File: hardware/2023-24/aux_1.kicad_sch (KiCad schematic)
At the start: 25 parts, among them J3 Screw_Terminal_01x04, Q5 BC817, U4 LM5066

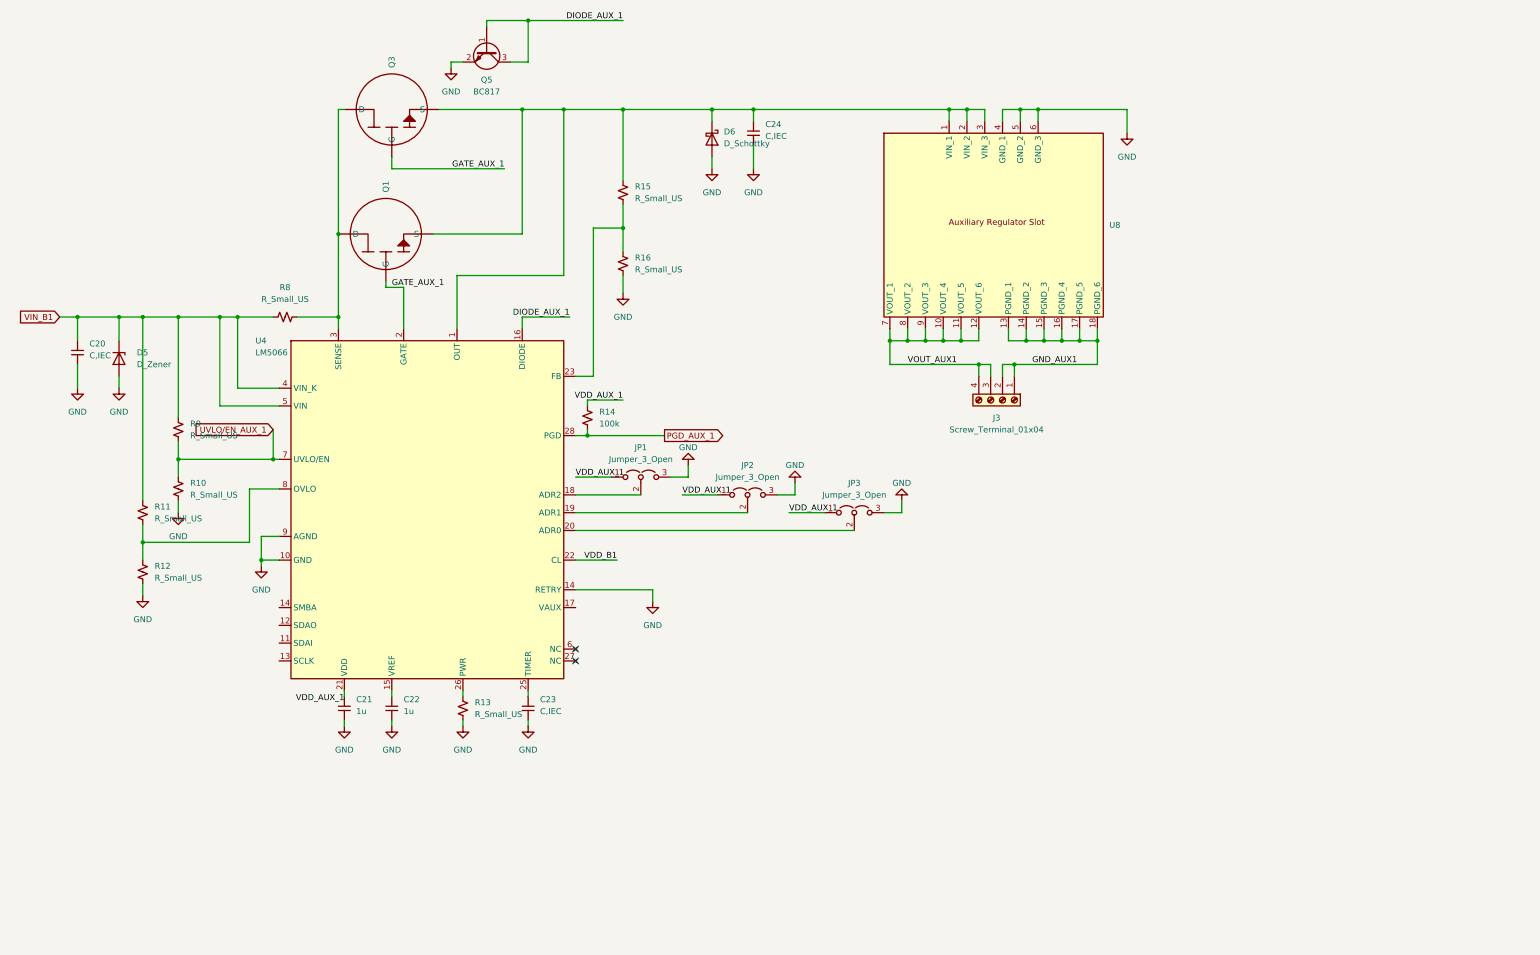
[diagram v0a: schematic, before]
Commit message: Pushing for design review
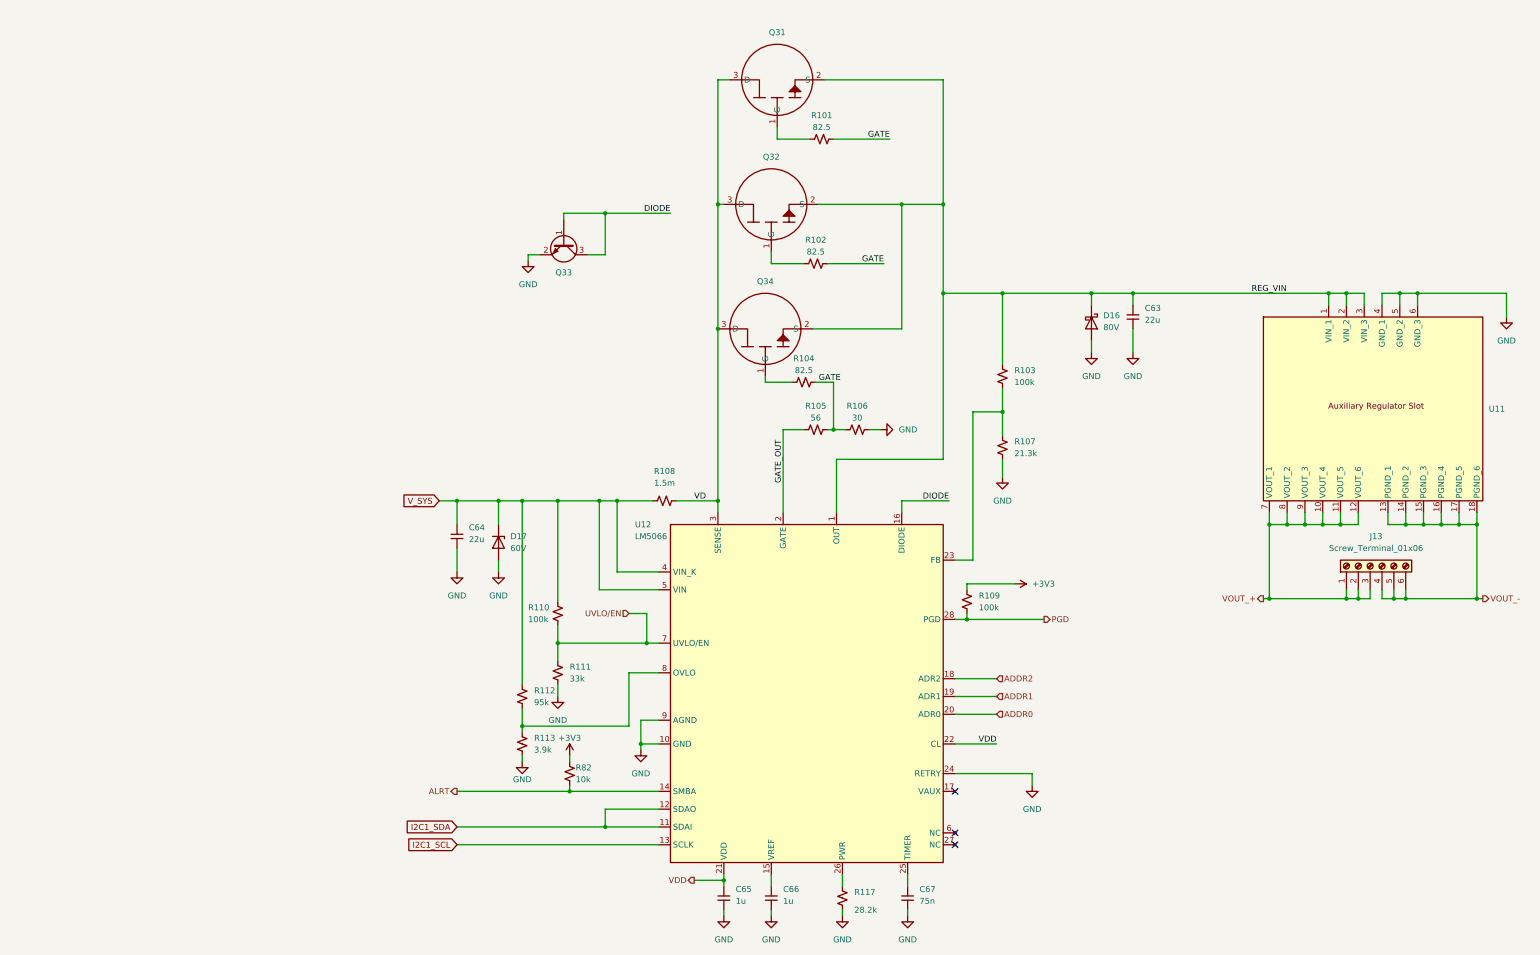
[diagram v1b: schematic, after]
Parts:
- removed C24: C,IEC, symbol PCM_Generic-50:C,IEC
- removed D5: D_Zener, symbol Device:D_Zener
- removed D6: D_Schottky, symbol Device:D_Schottky
- removed J3: Screw_Terminal_01x04, TerminalBlock:TerminalBlock_bornier-4_P5.08mm, symbol Connector:Screw_Terminal_01x04
- removed JP1, JP2, JP3: Jumper_3_Open, symbol Jumper:Jumper_3_Open
- removed Q5: BC817, Package_TO_SOT_SMD:SOT-23, symbol Transistor_BJT:BC817
- removed R10, R11, R12, R15, R16, R9: R_Small_US, symbol Device:R_Small_US
- added C63: 22u, Capacitor_SMD:CP_Elec_8x10, symbol PCM_Generic-50:C,IEC
- added D16: 80V, Diode_SMD:D_SMC, symbol Device:D_Schottky
- added D17: 60V, Diode_SMD:D_SMC, symbol Device:D_Zener
- added J13: Screw_Terminal_01x06, TerminalBlock_Phoenix:TerminalBlock_Phoenix_MKDS-1,5-6-5.08_1x06_P5.08mm_Horizontal, symbol Connector:Screw_Terminal_01x06
- added Q31: ~, Nexperia:WLCSP-8, symbol Nexperia:GAN3R2-100CBE
- added Q33: ~, Package_TO_SOT_SMD:SOT-23, symbol Transistor_BJT:BC817
- added R101, R102, R104: 82.5, Resistor_SMD:R_0603_1608Metric, symbol Device:R_Small_US
- added R103, R110: 100k, Resistor_SMD:R_0603_1608Metric, symbol Device:R_Small_US
- added R105: 56, Resistor_SMD:R_2512_6332Metric, symbol Device:R_Small_US
- added R106: 30, Resistor_SMD:R_2512_6332Metric, symbol Device:R_Small_US
- added R107: 21.3k, Resistor_SMD:R_0603_1608Metric, symbol Device:R_Small_US
- added R111: 33k, Resistor_SMD:R_0603_1608Metric, symbol Device:R_Small_US
- added R112: 95k, Resistor_SMD:R_0603_1608Metric, symbol Device:R_Small_US
- added R113: 3.9k, Resistor_SMD:R_0603_1608Metric, symbol Device:R_Small_US
- added R82: 10k, Resistor_SMD:R_0603_1608Metric, symbol Device:R_Small_US
- C64: renamed from C20; value C,IEC -> 22u; footprint (none) -> Capacitor_SMD:CP_Elec_8x10; MPN (none) -> EEE-FK2A220V
- C65: renamed from C21; footprint (none) -> Capacitor_SMD:C_0603_1608Metric
- C66: renamed from C22; footprint (none) -> Capacitor_SMD:C_0603_1608Metric
- C67: renamed from C23; value C,IEC -> 75n; footprint (none) -> Capacitor_SMD:C_0402_1005Metric; MPN (none) -> GRM31C5C1H753JA01L
- Q32: renamed from Q3; symbol Nexperia:GAN3R2-100CBEAZ -> Nexperia:GAN3R2-100CBE
- Q34: renamed from Q1; symbol Nexperia:GAN3R2-100CBEAZ -> Nexperia:GAN3R2-100CBE
- R108: renamed from R8; value R_Small_US -> 1.5m; footprint (none) -> Resistor_SMD:R_2512_6332Metric; MPN (none) -> WSL25121L500FEA; Manufacturer (none) -> Vishay
- R109: renamed from R14; footprint (none) -> Resistor_SMD:R_0603_1608Metric
- R117: renamed from R13; value R_Small_US -> 28.2k; footprint (none) -> Resistor_SMD:R_0603_1608Metric
- renumbered U8 to U11, U4 to U12
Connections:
- net VDD_B1 is gone; now on net VDD: U12.22 (CL)
- net GND: now also U12.24 (RETRY), C63.2 (-), D16.2 (A), D17.2 (A), Q33.2 (E), R106.2, R107.2, R111.1, R113.1; no longer U12.14 (SMBA)
- net VDD: now reaches C65.1 (+), U12.21 (VDD)
- net at U12.8 (OVLO): now also R112.1, R113.2
- net REG_VIN: now reaches U11.1 (VIN_1), U11.2 (VIN_2), U11.3 (VIN_3), U12.1 (OUT)
- net REG_VIN: now also Q32.2 (S), Q34.2 (S), C63.1 (+), D16.1 (K), Q31.2 (S), R103.1; no longer Q32. (S), Q34. (S)
- net I2C1_SDA: now reaches U12.11 (SDAI)
- net I2C1_SDA: now also U12.12 (SDAO)
- net I2C1_SCL: now reaches U12.13 (SCLK)
- net ALRT: now reaches U12.14 (SMBA)
- net ALRT: now also R82.2
- net ADDR2: now reaches U12.18 (ADR2)
- net ADDR1: now reaches U12.19 (ADR1)
- net ADDR0: now reaches U12.20 (ADR0)
- net at U12.23 (FB): now also R103.2, R107.1
- net VD: now reaches R108.2, U12.3 (SENSE)
- net VD: now also Q32.3 (D), Q34.3 (D), Q31.3 (D); no longer Q32. (S), Q34. (S)
- net DIODE_AUX_1 renamed DIODE
- net DIODE: now also Q33.1 (B), Q33.3 (C)
- removed net GATE_AUX_1: Q32. (S), Q34. (S), U12.2 (GATE)
- net GND_AUX1 renamed VOUT_-
- net VOUT_-: now also J13.4 (Pin_4), J13.5 (Pin_5), J13.6 (Pin_6)
- net PGD_AUX_1 renamed PGD
- net UVLO/EN_AUX_1 renamed UVLO/EN
- net UVLO/EN: now also R110.2, R111.2
- net VDD_AUX_1 renamed +3V3
- net +3V3: now also R82.1
- net VIN_B1 renamed V_SYS
- net V_SYS: now also D17.1 (K), R110.1, R112.2
- net VOUT_AUX1 renamed VOUT_+
- net VOUT_+: now also J13.1 (Pin_1), J13.2 (Pin_2), J13.3 (Pin_3)
- new net: Q34.1 (G), R104.1
- new net: Q32.1 (G), R102.1
- new net: Q31.1 (G), R101.1
- new net GATE: R101.2, R102.2, R104.2, R105.2, R106.1
- new net GATE_OUT: R105.1, U12.2 (GATE)
- no-connect marks 2 -> 3
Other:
- company: (none) -> Boise State University
- title: (none) -> Bender 2024 Power Supply
- moved on the sheet: C64, C65, C66, C67, R108, R109, R117, U11, U12
